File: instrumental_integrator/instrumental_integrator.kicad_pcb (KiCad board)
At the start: 2 copper layers, 30 parts, among them CN1 282841-2, CN2 282841-2, J1 Conn_01x01_Socket, J2 SS-52400-003, J3 Conn_01x01_Socket, J4 Conn_01x01_Socket, J5 Conn_01x01_Socket, J6 Conn_01x01_Socket, J7 Conn_01x01_Socket, J8 Conn_01x01_Socket, Q1 2N7002, SW1 DSWB06LHGET, SW2 TS1603-TZ38HBM, SW3 SW_Nidec_CAS-120A1, SW4 SW_Nidec_CAS-120A1, U1 INA828IDR, U10 ADS8681RUM, U2 RH-0515D, U4 BAT54_C2926171, U5 BAT54_C2926171, U6 BAT54_C2926171, U7 BAT54_C2926171, U8 LM27762, U9 TLV2387DR

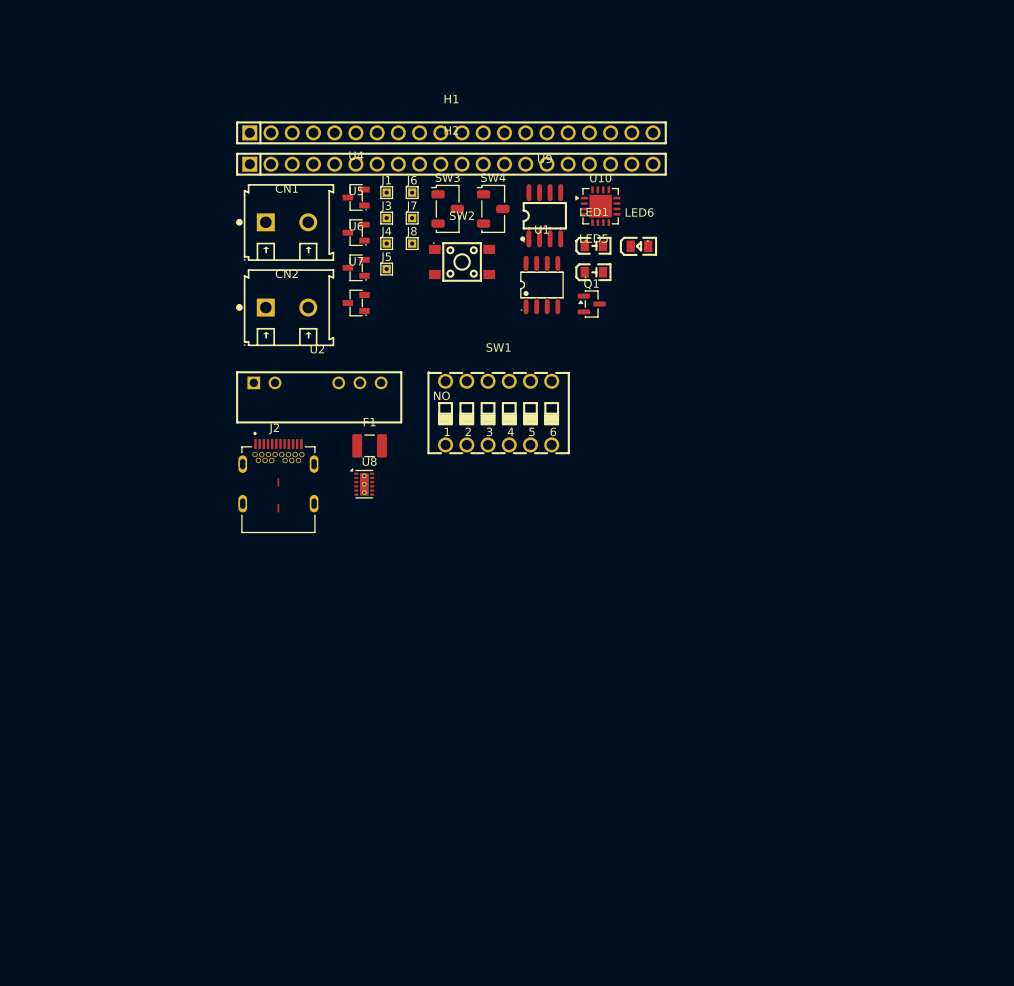
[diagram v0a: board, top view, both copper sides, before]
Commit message: started pcb
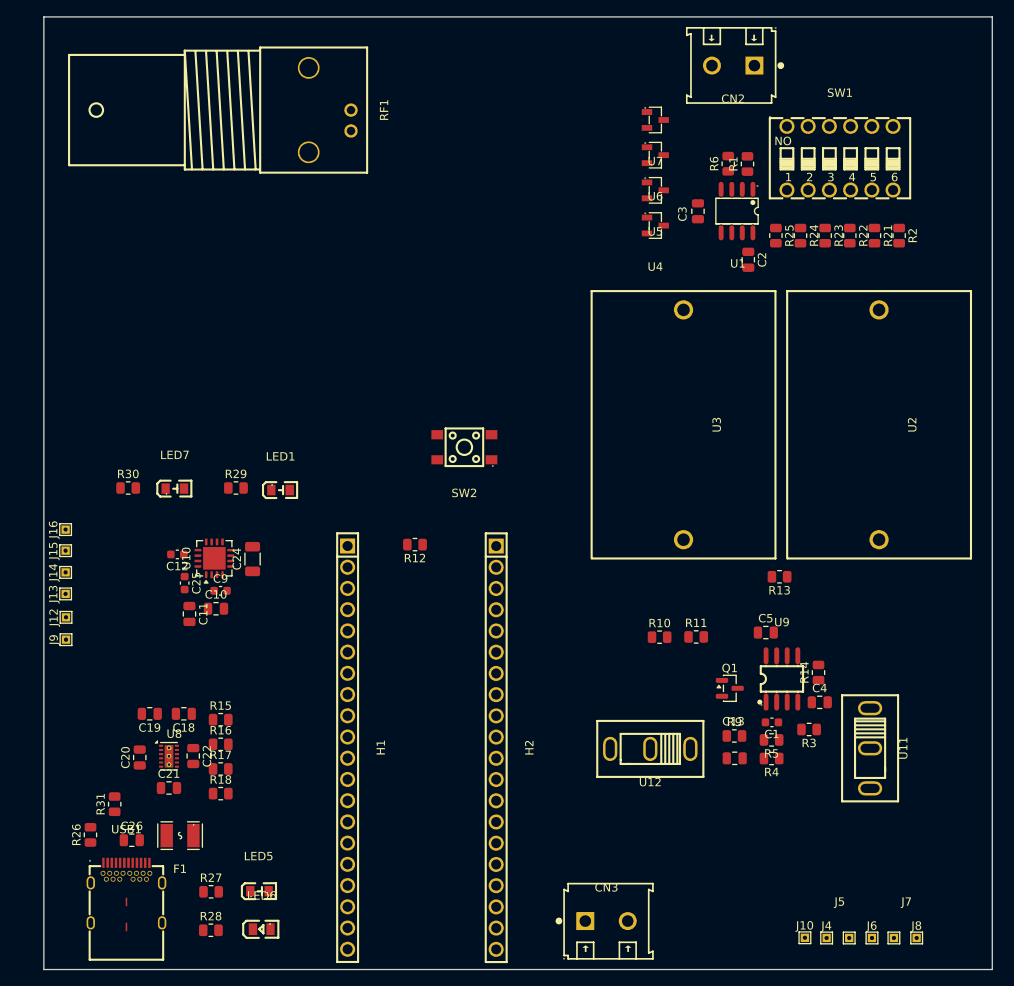
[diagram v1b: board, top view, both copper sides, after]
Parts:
- removed CN1: 282841-2, easyeda2kicad:CONN-TH_2P-P5.08_282841-2
- removed J1, J3: Conn_01x01_Socket, TestPoint:TestPoint_THTPad_1.0x1.0mm_Drill0.5mm
- removed J2: SS-52400-003, SS-52400-003:BELFUSE_SS-52400-003
- removed SW3, SW4: SW_Nidec_CAS-120A1, Button_Switch_SMD:Nidec_Copal_CAS-120A
- added C1: 10n, Capacitor_SMD:C_0603_1608Metric, F.Cu at (119.6, 130.4)
- added C10: 10uF, Capacitor_SMD:C_0805_2012Metric, F.Cu at (53.1, 116.8)
- added C11: 4.7uF, Capacitor_SMD:C_0805_2012Metric, F.Cu at (49.9, 117.5)
- added C12: 1uF, Capacitor_SMD:C_0603_1608Metric, F.Cu at (48.5, 110.3)
- added C13: 2.2n, Capacitor_SMD:C_0805_2012Metric, F.Cu at (115.2, 134.7)
- added C18: 2.2u, Capacitor_SMD:C_0805_2012Metric, F.Cu at (49.2, 129.4)
- added C19: 2.2u, Capacitor_SMD:C_0805_2012Metric, F.Cu at (45.2, 129.4)
- added C2: 100n, Capacitor_SMD:C_0805_2012Metric, F.Cu at (116.8, 75.1)
- added C20: 4.7u, Capacitor_SMD:C_0805_2012Metric, F.Cu at (44.0, 134.6)
- added C21: 4.7u, Capacitor_SMD:C_0805_2012Metric, F.Cu at (47.5, 138.3)
- added C22: 1u, Capacitor_SMD:C_0805_2012Metric, F.Cu at (50.4, 134.4)
- added C24: 22nF, Capacitor_SMD:C_1206_3216Metric, F.Cu at (57.5, 110.9)
- added C25: 1uF, Capacitor_SMD:C_0603_1608Metric, F.Cu at (49.4, 113.8)
- added C26: 0.1u, Capacitor_SMD:C_0805_2012Metric, F.Cu at (43.0, 144.5)
- added C3: 100n, Capacitor_SMD:C_0805_2012Metric, F.Cu at (110.8, 69.3)
- added C4: 100n, Capacitor_SMD:C_0805_2012Metric, F.Cu at (125.3, 128.0)
- added C5: 100n, Capacitor_SMD:C_0805_2012Metric, F.Cu at (118.9, 119.7)
- added C9: 1uF, Capacitor_SMD:C_0603_1608Metric, F.Cu at (53.6, 114.7)
- added CN3: 282841-2, easyeda2kicad:CONN-TH_2P-P5.08_282841-2, F.Cu at (99.8, 154.2)
- added J10: Conn_01x01_Socket, TestPoint:TestPoint_THTPad_1.0x1.0mm_Drill0.5mm, F.Cu at (123.6, 156.2)
- added J12: Conn_01x01_Socket, TestPoint:TestPoint_THTPad_1.0x1.0mm_Drill0.5mm, F.Cu at (35.1, 117.8)
- added J13: Conn_01x01_Socket, TestPoint:TestPoint_THTPad_1.0x1.0mm_Drill0.5mm, F.Cu at (35.1, 115.0)
- added J14: Conn_01x01_Socket, TestPoint:TestPoint_THTPad_1.0x1.0mm_Drill0.5mm, F.Cu at (35.1, 112.5)
- added J15: Conn_01x01_Socket, TestPoint:TestPoint_THTPad_1.0x1.0mm_Drill0.5mm, F.Cu at (35.1, 109.9)
- added J16: Conn_01x01_Socket, TestPoint:TestPoint_THTPad_1.0x1.0mm_Drill0.5mm, F.Cu at (35.1, 107.3)
- added J9: Conn_01x01_Socket, TestPoint:TestPoint_THTPad_1.0x1.0mm_Drill0.5mm, F.Cu at (35.1, 120.5)
- added LED7: LTST-C170TBKT, easyeda2kicad:LED0805-RD_BLUE, F.Cu at (48.2, 102.5)
- added R1: 5k, Resistor_SMD:R_0805_2012Metric, F.Cu at (116.7, 63.6)
- added R10: 100, Resistor_SMD:R_0805_2012Metric, F.Cu at (106.2, 120.2)
- added R11: 100k, Resistor_SMD:R_0805_2012Metric, F.Cu at (110.6, 120.2)
- added R12: 10k, Resistor_SMD:R_0805_2012Metric, F.Cu at (76.9, 109.2)
- added R13: 50.5k, Resistor_SMD:R_0805_2012Metric, F.Cu at (120.5, 113.0)
- added R14: 14.8k, Resistor_SMD:R_0805_2012Metric, F.Cu at (125.2, 124.5)
- added R15: 50.5k, Resistor_SMD:R_0805_2012Metric, F.Cu at (53.7, 130.1)
- added R16: 50.5k, Resistor_SMD:R_0805_2012Metric, F.Cu at (53.7, 133.1)
- added R17: 54.2k, Resistor_SMD:R_0805_2012Metric, F.Cu at (53.7, 136.0)
- added R18: 54.2k, Resistor_SMD:R_0805_2012Metric, F.Cu at (53.7, 138.9)
- added R2: 2k, Resistor_SMD:R_0805_2012Metric, F.Cu at (134.8, 72.2)
- added R21: 500, Resistor_SMD:R_0805_2012Metric, F.Cu at (131.9, 72.2)
- added R22: 120, Resistor_SMD:R_0805_2012Metric, F.Cu at (128.9, 72.2)
- added R23: 120, Resistor_SMD:R_0805_2012Metric, F.Cu at (126.0, 72.2)
- added R24: 120, Resistor_SMD:R_0805_2012Metric, F.Cu at (123.0, 72.2)
- added R25: 120, Resistor_SMD:R_0805_2012Metric, F.Cu at (120.1, 72.2)
- added R26: 5.1k, Resistor_SMD:R_0805_2012Metric, F.Cu at (38.1, 143.9)
- added R27: 50, Resistor_SMD:R_0805_2012Metric, F.Cu at (52.5, 150.7)
- added R28: 50, Resistor_SMD:R_0805_2012Metric, F.Cu at (52.5, 155.3)
- added R29: 300, Resistor_SMD:R_0805_2012Metric, F.Cu at (55.5, 102.4)
- added R3: 15k, Resistor_SMD:R_0805_2012Metric, F.Cu at (124.1, 131.3)
- added R30: 50, Resistor_SMD:R_0805_2012Metric, F.Cu at (42.6, 102.4)
- added R31: 5.1k, Resistor_SMD:R_0805_2012Metric, F.Cu at (41.0, 140.2)
- added R4: 10k, Resistor_SMD:R_0805_2012Metric, F.Cu at (119.6, 134.8)
- added R5: 1M, Resistor_SMD:R_0805_2012Metric, F.Cu at (119.6, 132.5)
- added R6: 5k, Resistor_SMD:R_0805_2012Metric, F.Cu at (114.4, 63.6)
- added R9: 1k, Resistor_SMD:R_0805_2012Metric, F.Cu at (115.1, 132.1)
- added RF1: KH-BNC50-3511, easyeda2kicad:ANT-TH_KH-BNC50-3511, F.Cu at (66.7, 57.1)
- added U11: SS12D10G5, easyeda2kicad:SW-TH_SHOU-HAN_SS12D10G4, F.Cu at (131.4, 133.5)
- added U12: SS12D10G5, easyeda2kicad:SW-TH_SHOU-HAN_SS12D10G4, F.Cu at (105.1, 133.6)
- added U3: C3D22UF500V82CB0300, easyeda2kicad:CAP-TH_L32.0-W22.0-P27.50-D1.3, F.Cu at (109.0, 94.8)
- added USB1: SS-52400-003, easyeda2kicad:TYPE-C-SMD_SS-52400-003, F.Cu at (42.4, 151.1)
- F1: footprint 0ZCH0110AF2E:FUSC3225X100N -> easyeda2kicad:F1210
- U2: value RH-0515D -> C3D22UF500V82CB0300; footprint easyeda2kicad:PWRM-TH_5P-L19.7-W6.0-P2.54_RH-051509D -> easyeda2kicad:CAP-TH_L32.0-W22.0-P27.50-D1.3
- moved J6 104.8 mm to (131.6, 156.2)
- moved J7 103.7 mm to (134.2, 156.2)
- moved J8 102.7 mm to (136.9, 156.2)
- moved J4 98.4 mm to (126.2, 156.2)
- moved J5 97.3 mm to (128.9, 156.2)
- moved LED6 93.4 mm to (58.6, 155.2)
- moved LED5 84.2 mm to (58.3, 150.6)
- moved H1 74.6 mm to (68.8, 133.4), turned to -90 degrees
- moved H2 70.0 mm to (86.6, 133.5), turned to -90 degrees
- moved U2 67.4 mm to (132.4, 94.8), turned to -90 degrees
- moved U10 62.5 mm to (52.9, 110.8), turned to 90 degrees
- moved U9 62.3 mm to (120.8, 125.2)
- moved CN2 60.7 mm to (115.0, 51.8), turned to 180 degrees
- moved F1 51.9 mm to (48.8, 144.0), turned to 180 degrees
- moved SW1 51.0 mm to (127.8, 62.9)
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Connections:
- U2 pad 1: +5V -> Net-(U1-OUT)
- U2 pad 2: GND -> /gain_out
- U9 pad 2: Net-(U9A-IN1-) -> /opin-
- U9 pad 3: Net-(U9A-IN1+) -> /opin+
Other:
- board outline added: 113.5 x 114 mm
- copper layers 2 -> 4

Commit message: finished pcb design V1
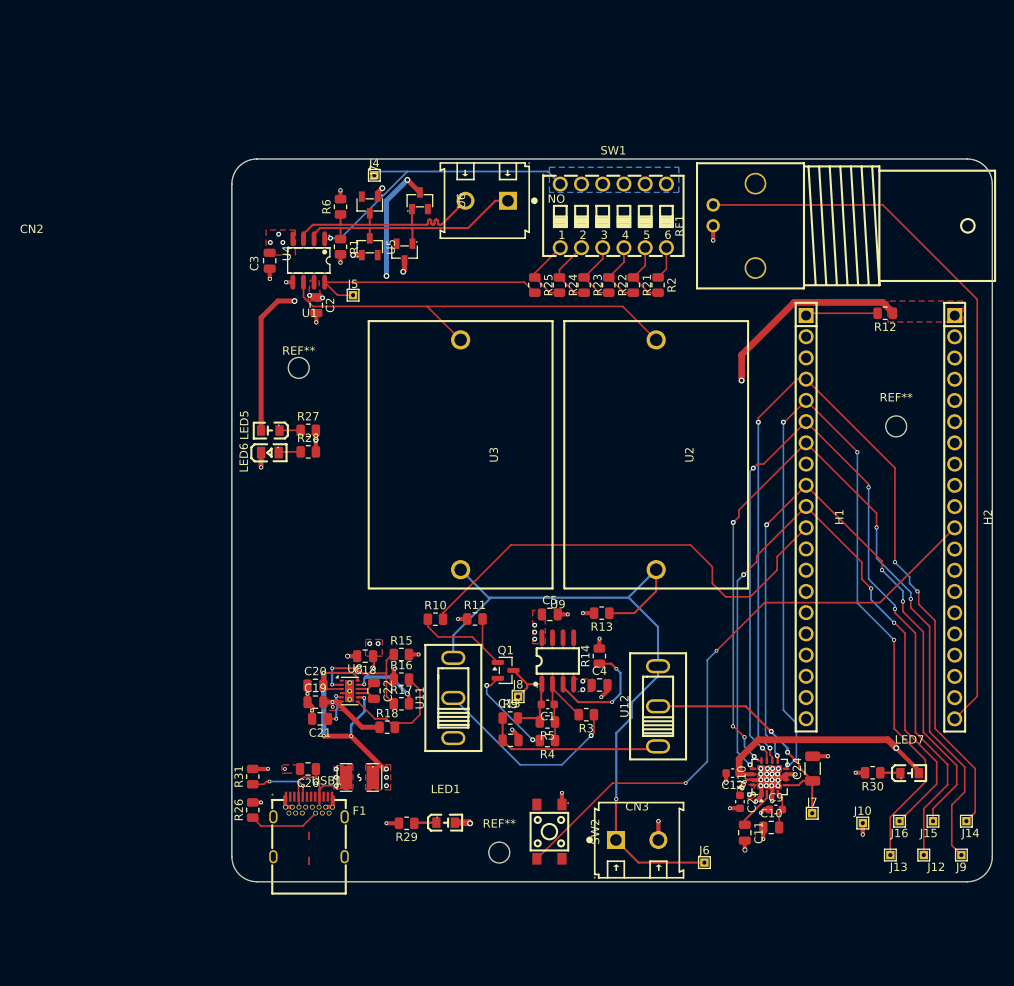
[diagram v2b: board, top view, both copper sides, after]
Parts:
- added REF**: MountingHole_2.5mm, MountingHole:MountingHole_2.5mm, F.Cu at (134.5, 95.0)
- added REF**: MountingHole_2.5mm, MountingHole:MountingHole_2.5mm, F.Cu at (87.0, 146.0)
- added REF**: MountingHole_2.5mm, MountingHole:MountingHole_2.5mm, F.Cu at (63.0, 88.0)
- moved J14 111.8 mm to (142.9, 142.2), turned to 180 degrees
- moved J9 110.2 mm to (142.3, 146.3), turned to 180 degrees
- moved J15 108.7 mm to (138.9, 142.2), turned to 180 degrees
- moved J12 106.5 mm to (137.8, 146.3), turned to 180 degrees
- moved J4 106.1 mm to (72.0, 65.0)
- moved J16 105.7 mm to (134.9, 142.2), turned to 180 degrees
- moved J13 103.5 mm to (133.8, 146.3), turned to 180 degrees
- moved J5 97.2 mm to (69.5, 79.3)
- moved R30 95.4 mm to (131.7, 136.4), turned to 180 degrees
- moved LED7 94.3 mm to (136.1, 136.5)
- moved C24 71.6 mm to (124.5, 135.9)
- moved C11 71.4 mm to (116.4, 143.6)
- moved C10 71.4 mm to (119.5, 143.0)
- moved C12 71.4 mm to (114.9, 136.5)
- moved C25 71.4 mm to (115.8, 139.9)
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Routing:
- net /GP2: track 0.00 -> 111.1 mm, vias 0 -> 4
- net /GP3: track 0.00 -> 108.7 mm, vias 0 -> 4
- net /GP4: track 0.00 -> 104.7 mm, vias 0 -> 4
- net /GP5: track 0.00 -> 101.7 mm, vias 0 -> 6
- net /gain_out: track 0.00 -> 88.8 mm, vias 0 -> 1
- net /GP16: track 0.00 -> 87.6 mm
- net /GP6: track 0.00 -> 84.4 mm, vias 0 -> 4
- net /GP7: track 0.00 -> 81.6 mm, vias 0 -> 4
- net /RUN: track 0.00 -> 73.5 mm, vias 0 -> 2
- net GND: track 0.00 -> 65.0 mm, vias 0 -> 52
- net +5V: track 0.00 -> 58.0 mm, vias 0 -> 11
- net /GP8: track 0.00 -> 55.7 mm
- net Net-(U1-OUT): track 0.00 -> 51.8 mm
- net +2V5: track 0.00 -> 46.2 mm, vias 0 -> 14
- net /rg1: track 0.00 -> 36.3 mm, vias 0 -> 1
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- added copper zone on F.Cu, net +2V5
- added copper zone on In1.Cu, net +2V5
- added copper zone on In1.Cu, net +3.3V
- added copper zone on F.Cu, net +5V
- added copper zone on In1.Cu, net +5V
- added copper zone on F.Cu, net -2V5
- added copper zone on In1.Cu, net -2V5
- added copper zone on F.Cu, net /power/VBUS
- added copper zone on In1.Cu, net /power/VBUS
- added copper zone on B.Cu, net /rg1
- added copper zone on F.Cu, net GND
- added copper zone on In2.Cu, net GND
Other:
- board size 113.5 x 114 mm -> 91 x 86.5 mm
